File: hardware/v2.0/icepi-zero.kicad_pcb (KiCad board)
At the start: 4 copper layers, 65 x 30 mm, 193 parts, among them IC1 IS42S16160J-6BLI, IC2 LTC2256CUJ-12#PBF, J1 Conn_02x20_Counter_Clockwise, J2 GPDI_C_1.3, J3 USB_C_Receptacle_USB2.0_14P, J4 USB_C_Receptacle_USB2.0_14P, J5 USB_C_Receptacle_USB2.0_14P, J6 Micro_SD_Card_Det2, J7 RSP-122811-01, SW1 SW_Push, SW2 SW_Push, U1 ECP5U-25F-CABGA256, U10 TPD2EUSB30A, U11 LT1993CUD-2_PBF, U12 W25Q128JVS, U2 LTC3407AEDD-2_PBF, U3 TLV62569DBV, U4 LP5912-1.8DRV, U5 TPD2EUSB30A, U6 PCA9306DC1, U7 TPD2EUSB30A, U8 TPD2EUSB30A, U9 FT231XQ, Y1 SG-8018CG 50.000000MHz, Y2 SG-8018CG 50.000000MHz

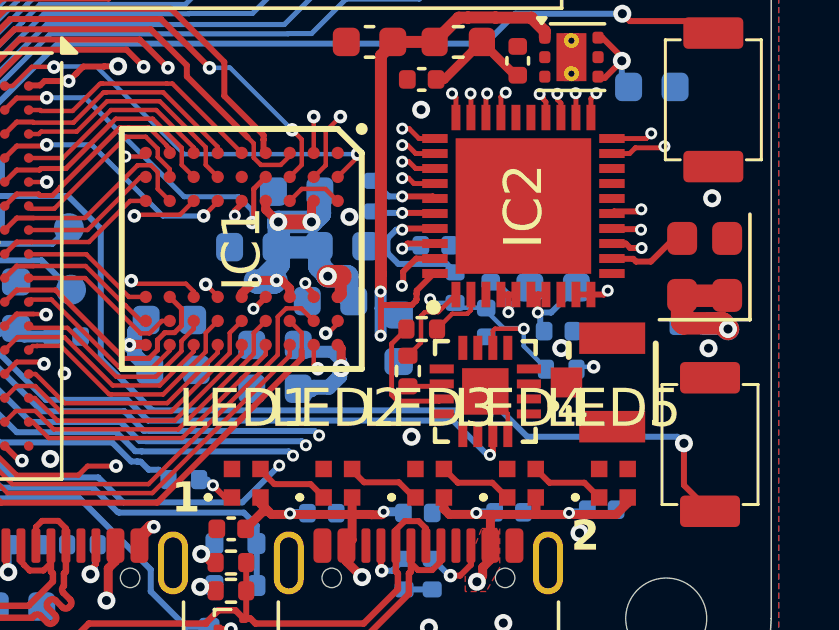
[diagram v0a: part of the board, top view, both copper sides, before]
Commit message: DRC almost pass
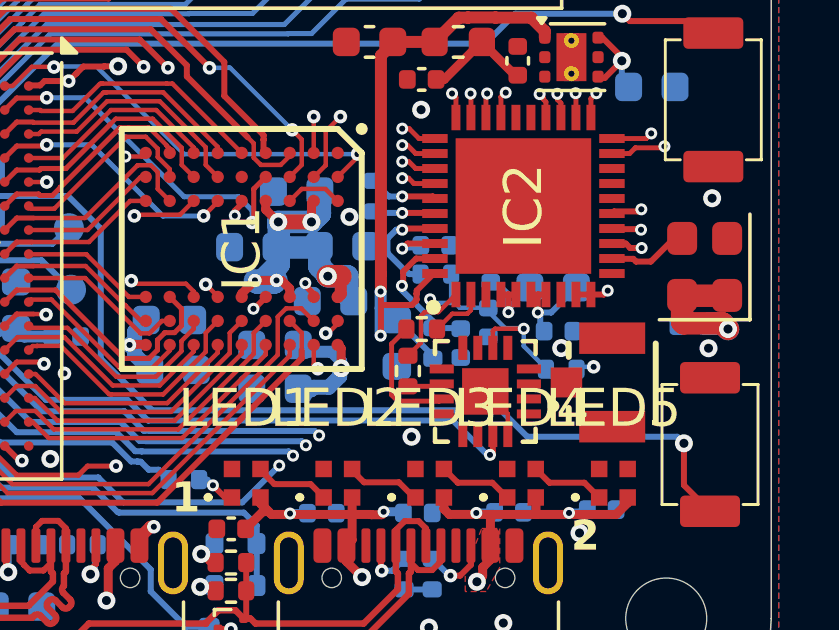
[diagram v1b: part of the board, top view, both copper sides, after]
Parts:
- added C74: 1u, Capacitor_SMD:C_0402_1005Metric, B.Cu at (170.4, 107.3)
- added R5: 1k, Resistor_SMD:R_0402_1005Metric, B.Cu at (169.5, 107.3)
- moved R52 0.78 mm to (169.6, 105.0), turned to 0 degrees
- moved C64 0.17 mm to (168.3, 107.3)
- moved C69 0.07 mm to (171.3, 106.6)
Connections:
- R52 pad 1: /ADC/VOCM -> Net-(IC2-VCM)
- R52 pad 2: Net-(IC2-VCM) -> /ADC/VOCM
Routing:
- net /ADC/SENSE: track 23.9 -> 26.7 mm
- net +1V8: track 29.6 -> 31.1 mm
- net Net-(IC2-VCM): track 4.72 -> 3.60 mm
- net /ADC/VOCM: track 6.82 -> 7.79 mm
- net GND: vias 100 -> 98
- net /ADC/CLKOUT-: vias 0 -> 2
